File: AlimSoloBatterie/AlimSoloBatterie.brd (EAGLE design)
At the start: 36.8 x 40.3 mm, 13 parts

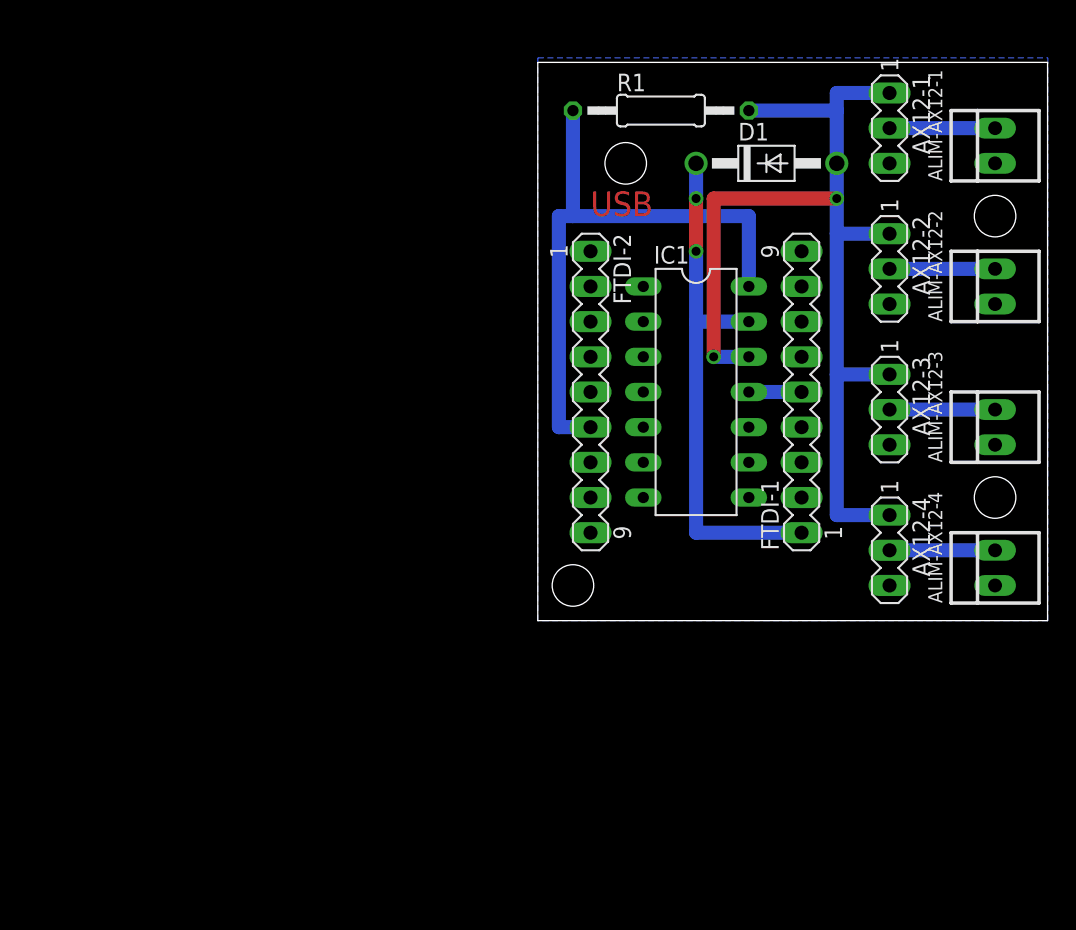
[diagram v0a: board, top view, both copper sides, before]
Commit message: Cleaning and new cards
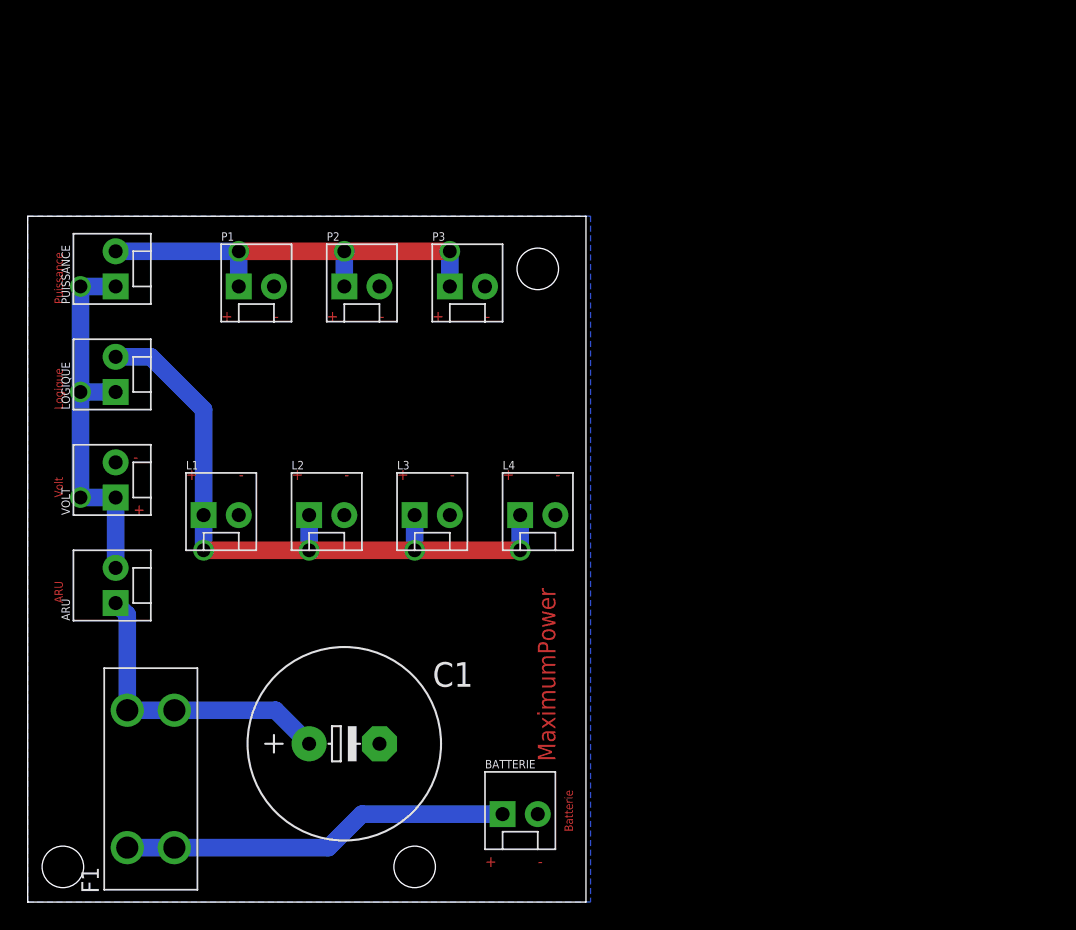
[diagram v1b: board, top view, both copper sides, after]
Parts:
- removed ALIM-AX12-1, ALIM-AX12-2, ALIM-AX12-3, ALIM-AX12-4: 22-23-2021, con-molex:22-23-2021
- removed AX12-1, AX12-2, AX12-3, AX12-4: (no value), con-lstb:MA03-1
- removed D1: 1N4004, diode:DO41-10
- removed FTDI-1, FTDI-2: (no value), con-lstb:MA09-1
- removed IC1: (no value), ic-package:DIL14
- removed R1: 10k, rcl:0207/12
- added ARU, BATTERIE, L1, L2, L3, L4, LOGIQUE, P1, P2, P3, PUISSANCE, VOLT: (no value), SparkFun-Connectors:MOLEX-1X2
- added C1: (no value), rcl:E5-13
- added F1: 3568, CarFuseHolder:FUSE_3568
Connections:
- removed net 5V: FTDI-2.6, IC1.14, R1.1
- removed net AX12-DATA: AX12-1.1, AX12-2.1, AX12-3.1, AX12-4.1, D1.A, IC1.12, R1.2
- removed net RXD: FTDI-1.5, IC1.11
- removed net TXD: D1.C, FTDI-1.1, IC1.13
- new net N$5: L1.1, L2.1, L3.1, L4.1, LOGIQUE.2
- net GND: now also BATTERIE.2, C1.-, L1.2, L2.2, L3.2, L4.2, P1.2, P2.2, P3.2, VOLT.2; no longer ALIM-AX12-1.1, ALIM-AX12-2.1, ALIM-AX12-3.1, ALIM-AX12-4.1, AX12-1.3, AX12-2.3, AX12-3.3, AX12-4.3, FTDI-1.7, IC1.7
- net N$1: now also BATTERIE.1, F1.1, F1.3; no longer ALIM-AX12-4.2, AX12-4.2
- net N$2: now also ARU.1, C1.+, F1.2, F1.4; no longer ALIM-AX12-3.2, AX12-3.2
- net N$3: now also ARU.2, LOGIQUE.1, PUISSANCE.1, VOLT.1; no longer ALIM-AX12-2.2, AX12-2.2
- net N$4: now also P1.1, P2.1, P3.1, PUISSANCE.2; no longer ALIM-AX12-1.2, AX12-1.2
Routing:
- net AX12-DATA: track 74.9 -> 0.00 mm, vias 2 -> 0
- net N$5: track 0.00 -> 48.6 mm, vias 0 -> 4
- net 5V: track 43.9 -> 0.00 mm
- net TXD: track 38.1 -> 0.00 mm, vias 2 -> 0
- net N$4: track 7.62 -> 31.7 mm, vias 0 -> 3
- net N$1: track 7.62 -> 28.3 mm
- net N$3: track 7.62 -> 27.9 mm, vias 0 -> 3
- net N$2: track 7.62 -> 22.2 mm
- net RXD: track 3.81 -> 0.00 mm
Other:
- board size 36.8 x 40.3 mm -> 40.3 x 49.5 mm
- board text added: "+"
- board text added: "-"
- board text added: "ARU"
- board text added: "Batterie"
- board text added: "Logique"
- board text added: "MaximumPower"
- board text added: "Puissance"
- board text added: "Volt"
- board text removed: "USB"
